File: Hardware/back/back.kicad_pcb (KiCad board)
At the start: 2 copper layers, 103 x 49.6 mm, 2 parts, among them J1 Conn_01x06_Male

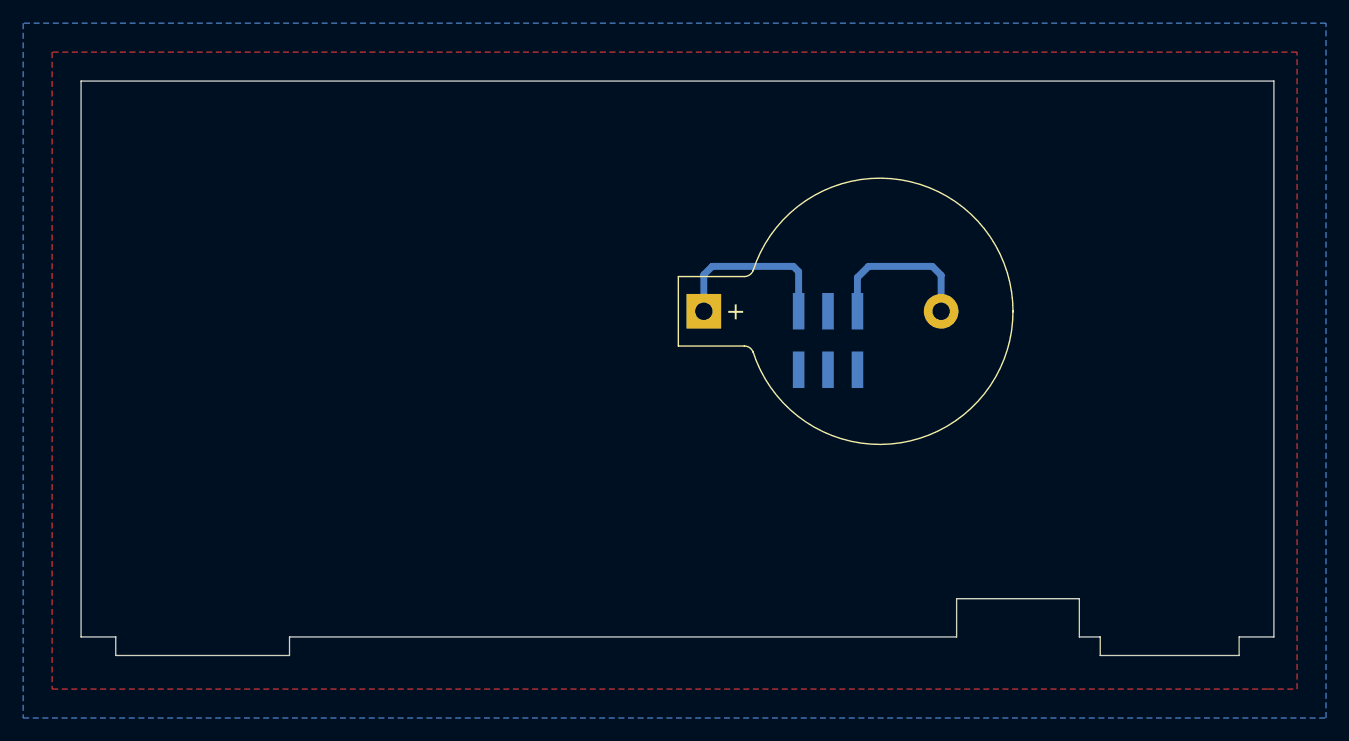
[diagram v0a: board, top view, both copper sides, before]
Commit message: Major HW and FW improvements
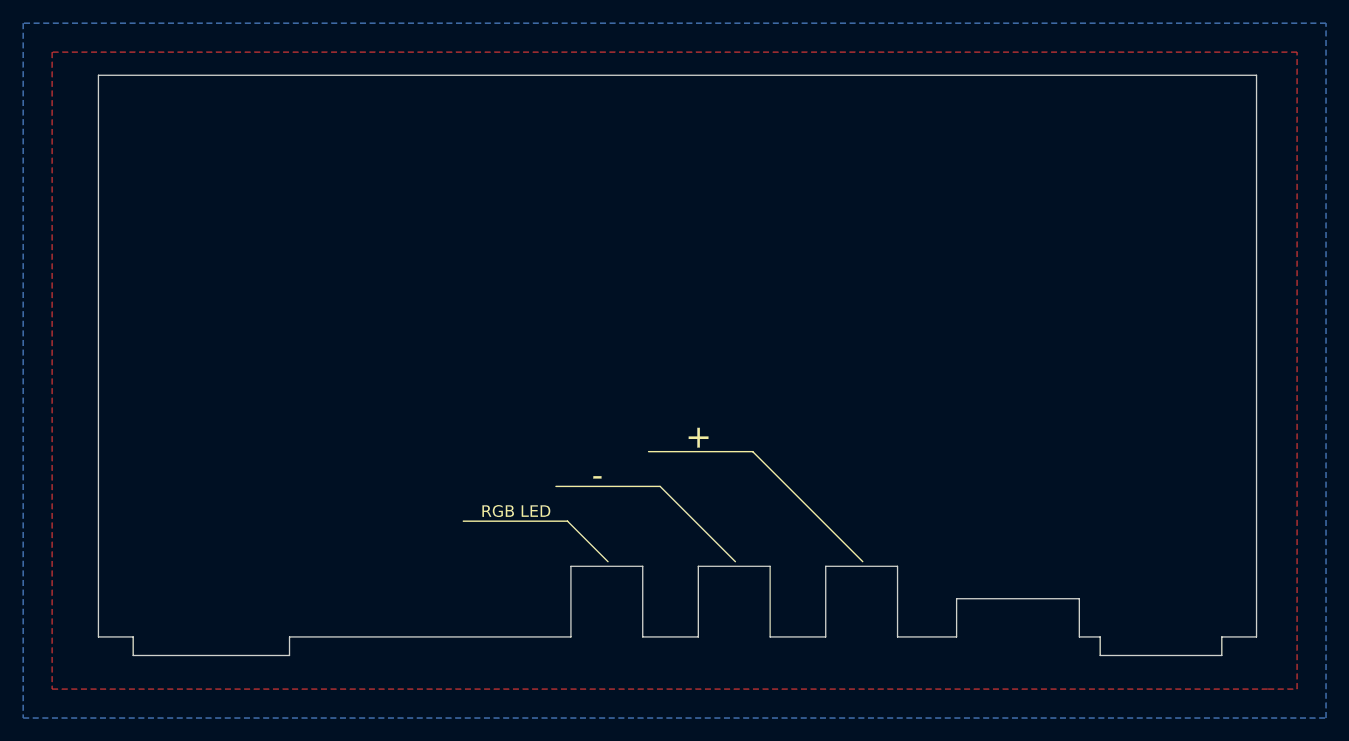
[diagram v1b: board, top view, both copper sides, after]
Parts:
- removed BT1: Battery_Cell, Battery:BatteryHolder_Keystone_103_1x20mm
- removed J1: Conn_01x06_Male, Connector_PinHeader_2.54mm:PinHeader_2x03_P2.54mm_Vertical_SMD
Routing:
- net Net-(BT1-Pad1): track 15.2 -> 0.00 mm
- net Net-(BT1-Pad2): track 14.0 -> 0.00 mm
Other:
- board size 103 x 49.6 mm -> 100 x 50.1 mm
- rule pad_to_mask_clearance: 0.051 -> 0
- board text added: "+"
- board text added: "-"
- board text added: "RGB LED"
